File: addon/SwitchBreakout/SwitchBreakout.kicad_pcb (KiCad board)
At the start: 2 copper layers, 127.8 x 194.6 mm, 209 parts, among them IC1 SN74HCS72QPWRQ1, IC10 SN74HCS72QPWRQ1, IC11 SN74HCS72QPWRQ1, IC12 SN74HCS72QPWRQ1, IC13 SN74HCS72QPWRQ1, IC14 SN74HCS72QPWRQ1, IC15 SN74HCS72QPWRQ1, IC16 SN74HCS72QPWRQ1, IC2 SN74HCS72QPWRQ1, IC3 SN74HCS72QPWRQ1, IC4 SN74HCS72QPWRQ1, IC5 SN74HCS72QPWRQ1, IC6 SN74HCS72QPWRQ1, IC7 SN74HCS72QPWRQ1, IC8 SN74HCS72QPWRQ1, IC9 SN74HCS72QPWRQ1, J1 SS73100-047F, J2 Conn_02x20_Odd_Even, J3 Conn_02x20_Odd_Even, J6 SS73100-047F, J7 SS73100-047F

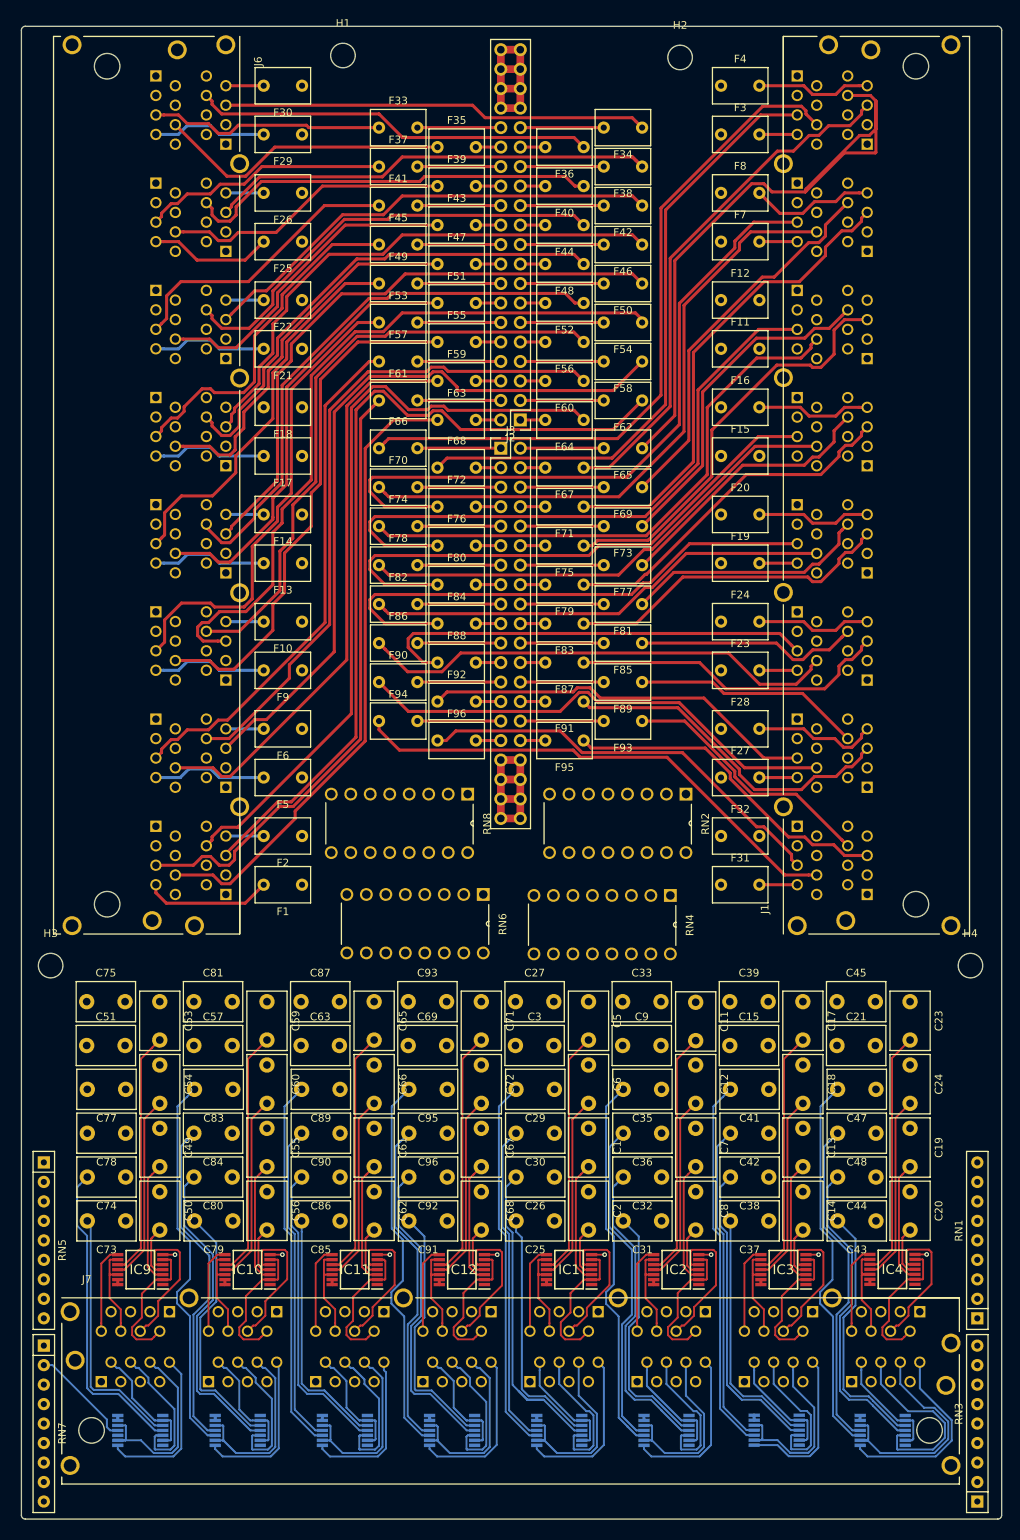
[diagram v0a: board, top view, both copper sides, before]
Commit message: UP
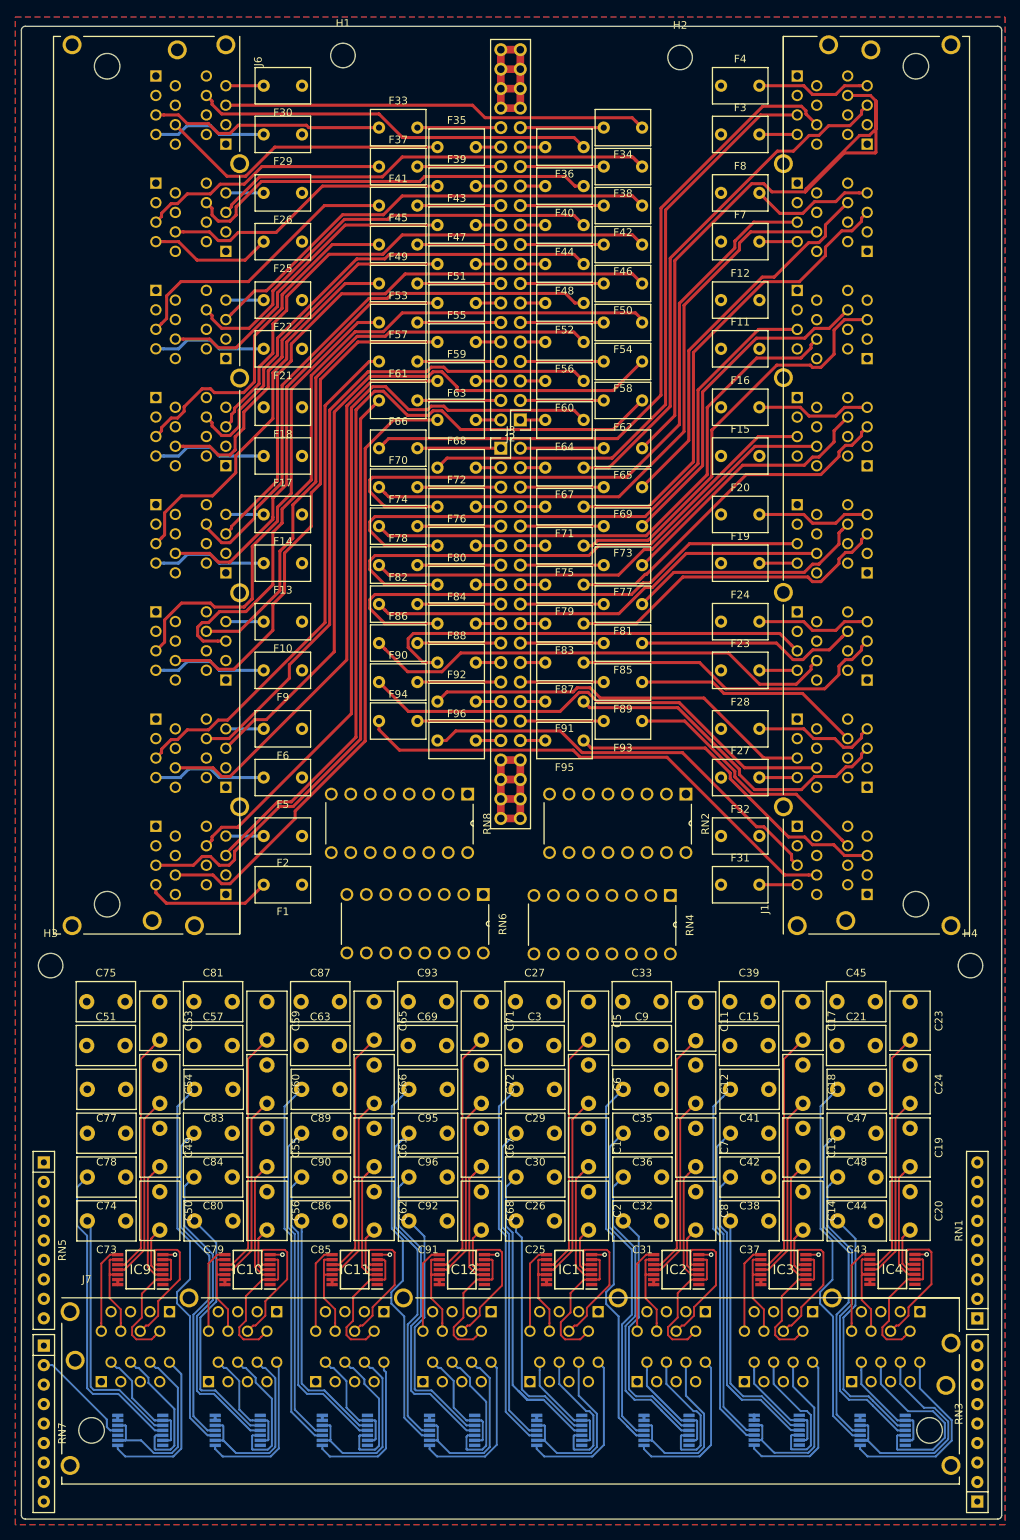
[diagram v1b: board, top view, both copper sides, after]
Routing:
- added copper zone on F.Cu, net GND
- added copper zone on B.Cu, net VCC
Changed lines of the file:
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@@
     (thickness 1.6)
     (drawings 8)
-    (tracks 1933)
+    (tracks 1932)
     (zones 0)
     (modules 209)
@@
   (segment (start 200.682511 194.200009) (end 200.682511 198.169991) (width 0.25) (layer B.Cu) (net 40))
   (segment (start 195.834 187.325) (end 195.834 190.169722) (width 0.25) (layer B.Cu) (net 40))
-  (segment (start 193.294 198.135) (end 196.349678 198.135) (width 0.25) (layer B.Cu) (net 41))
   (segment (start 201.652999 188.063999) (end 200.914 187.325) (width 0.25) (layer B.Cu) (net 41))
-  (segment (start 200.540303 199.585019) (end 201.652999 198.472323) (width 0.25) (layer B.Cu) (net 41))
   (segment (start 201.652999 198.472323) (end 201.652999 188.063999) (width 0.25) (layer B.Cu) (net 41))
-  (segment (start 197.799698 199.58502) (end 200.540303 199.585019) (width 0.25) (layer B.Cu) (net 41))
-  (segment (start 196.349678 198.135) (end 197.799698 199.58502) (width 0.25) (layer B.Cu) (net 41))
+  (segment (start 193.294 198.61) (end 193.294 198.135) (width 0.25) (layer B.Cu) (net 41))
+  (segment (start 194.269019 199.585019) (end 193.294 198.61) (width 0.25) (layer B.Cu) (net 41))
+  (segment (start 200.540303 199.585019) (end 194.269019 199.585019) (width 0.25) (layer B.Cu) (net 41))
+  (segment (start 201.652999 198.472323) (end 200.540303 199.585019) (width 0.25) (layer B.Cu) (net 41))
   (segment (start 194.2815 195.535) (end 193.294 195.535) (width 0.25) (layer B.Cu) (net 42))
   (segment (start 194.356501 195.610001) (end 194.2815 195.535) (width 0.25) (layer B.Cu) (net 42))
@@
   (segment (start 194.191502 197.485) (end 194.356501 197.320001) (width 0.25) (layer B.Cu) (net 42))
   (segment (start 193.294 197.485) (end 194.191502 197.485) (width 0.25) (layer B.Cu) (net 42))
-  (segment (start 198.374 188.370103) (end 198.374 187.325) (width 0.25) (layer B.Cu) (net 42))
-  (segment (start 198.374 190.5) (end 198.374 188.370103) (width 0.25) (layer B.Cu) (net 42))
-  (segment (start 201.132521 198.356391) (end 201.132521 193.258521) (width 0.25) (layer B.Cu) (net 42))
-  (segment (start 200.353902 199.13501) (end 201.132521 198.356391) (width 0.25) (layer B.Cu) (net 42))
-  (segment (start 197.986098 199.13501) (end 200.353902 199.13501) (width 0.25) (layer B.Cu) (net 42))
-  (segment (start 196.336088 197.485) (end 197.986098 199.13501) (width 0.25) (layer B.Cu) (net 42))
-  (segment (start 201.132521 193.258521) (end 198.374 190.5) (width 0.25) (layer B.Cu) (net 42))
-  (segment (start 193.294 197.485) (end 196.336088 197.485) (width 0.25) (layer B.Cu) (net 42))
+  (segment (start 194.2815 197.485) (end 193.294 197.485) (width 0.25) (layer B.Cu) (net 42))
+  (segment (start 195.931511 199.135011) (end 194.2815 197.485) (width 0.25) (layer B.Cu) (net 42))
+  (segment (start 200.353901 199.135011) (end 195.931511 199.135011) (width 0.25) (layer B.Cu) (net 42))
+  (segment (start 201.132521 198.356391) (end 200.353901 199.135011) (width 0.25) (layer B.Cu) (net 42))
+  (segment (start 201.132521 193.258521) (end 201.132521 198.356391) (width 0.25) (layer B.Cu) (net 42))
+  (segment (start 198.374 190.5) (end 201.132521 193.258521) (width 0.25) (layer B.Cu) (net 42))
+  (segment (start 198.374 187.325) (end 198.374 190.5) (width 0.25) (layer B.Cu) (net 42))
   (segment (start 179.314 188.370103) (end 179.314 187.325) (width 0.25) (layer B.Cu) (net 43))
   (segment (start 179.314 190.4145) (end 179.314 188.370103) (width 0.25) (layer B.Cu) (net 43))
@@
   (segment (start 118.634531 188.865531) (end 118.63453 198.572792) (width 0.25) (layer B.Cu) (net 69))
   (segment (start 117.094 187.325) (end 118.634531 188.865531) (width 0.25) (layer B.Cu) (net 69))
-  (segment (start 111.3335 197.515) (end 110.346 197.515) (width 0.25) (layer B.Cu) (net 70))
-  (segment (start 111.408501 197.439999) (end 111.3335 197.515) (width 0.25) (layer B.Cu) (net 70))
-  (segment (start 111.408501 195.640001) (end 111.408501 197.439999) (width 0.25) (layer B.Cu) (net 70))
+  (segment (start 118.184521 190.650799) (end 115.597721 188.063999) (width 0.25) (layer B.Cu) (net 70))
+  (segment (start 113.388088 197.515) (end 115.038099 199.165011) (width 0.25) (layer B.Cu) (net 70))
   (segment (start 111.3335 195.565) (end 111.408501 195.640001) (width 0.25) (layer B.Cu) (net 70))
-  (segment (start 110.346 195.565) (end 111.3335 195.565) (width 0.25) (layer B.Cu) (net 70))
-  (segment (start 118.184521 198.386391) (end 118.184521 190.650799) (width 0.25) (layer B.Cu) (net 70))
-  (segment (start 117.405902 199.16501) (end 118.184521 198.386391) (width 0.25) (layer B.Cu) (net 70))
   (segment (start 115.038099 199.165011) (end 117.405902 199.16501) (width 0.25) (layer B.Cu) (net 70))
+  (segment (start 111.408501 195.640001) (end 111.408501 197.439999) (width 0.25) (layer B.Cu) (net 70))
   (segment (start 115.292999 188.063999) (end 114.554 187.325) (width 0.25) (layer B.Cu) (net 70))
-  (segment (start 118.184521 190.650799) (end 115.597721 188.063999) (width 0.25) (layer B.Cu) (net 70))
-  (segment (start 113.388088 197.515) (end 115.038099 199.165011) (width 0.25) (layer B.Cu) (net 70))
-  (segment (start 115.597721 188.063999) (end 115.292999 188.063999) (width 0.25) (layer B.Cu) (net 70))
+  (segment (start 117.405902 199.16501) (end 118.184521 198.386391) (width 0.25) (layer B.Cu) (net 70))
+  (segment (start 110.346 195.565) (end 111.3335 195.565) (width 0.25) (layer B.Cu) (net 70))
+  (segment (start 111.408501 197.439999) (end 111.3335 197.515) (width 0.25) (layer B.Cu) (net 70))
+  (segment (start 118.184521 198.386391) (end 118.184521 190.650799) (width 0.25) (layer B.Cu) (net 70))
   (segment (start 110.346 197.515) (end 113.388088 197.515) (width 0.25) (layer B.Cu) (net 70))
+  (segment (start 115.597721 188.063999) (end 115.292999 188.063999) (width 0.25) (layer B.Cu) (net 70))
+  (segment (start 111.3335 197.515) (end 110.346 197.515) (width 0.25) (layer B.Cu) (net 70))
   (segment (start 127.605 194.915) (end 127.9345 194.915) (width 0.25) (layer B.Cu) (net 71))
   (segment (start 126.189999 193.499999) (end 127.605 194.915) (width 0.25) (layer B.Cu) (net 71))
@@
   (segment (start 194.552001 117.544999) (end 198.167001 121.159999) (width 0.4) (layer F.Cu) (net 386))
   (segment (start 170.874018 107.88002) (end 183.955018 107.88002) (width 0.4) (layer F.Cu) (net 386))
+  (zone (net 1) (net_name GND) (layer F.Cu) (hatch edge 0.508)
+    (connect_pads (clearance 0.508))
+    (min_thickness 0.254)
+    (fill (arc_segments 32) (thermal_gap 0.508) (thermal_bridge_width 0.508))
+    (polygon
+      (pts
+        (xy 226 208.5) (xy 97 208.5) (xy 97 12) (xy 226 12)
+      )
+    )
+  )
+  (zone (net 2) (net_name VCC) (layer B.Cu) (hatch edge 0.508)
+    (connect_pads (clearance 0.508))
+    (min_thickness 0.254)
+    (fill (arc_segments 32) (thermal_gap 0.508) (thermal_bridge_width 0.508))
+    (polygon
+      (pts
+        (xy 226 208.5) (xy 97 208.5) (xy 97 12) (xy 226 12)
+      )
+    )
+  )
 )
